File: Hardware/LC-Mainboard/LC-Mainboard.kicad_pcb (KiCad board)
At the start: 2 copper layers, 103 x 63 mm, 2 parts, among them J1 Raspberry_Pi, J2 Charge Controller

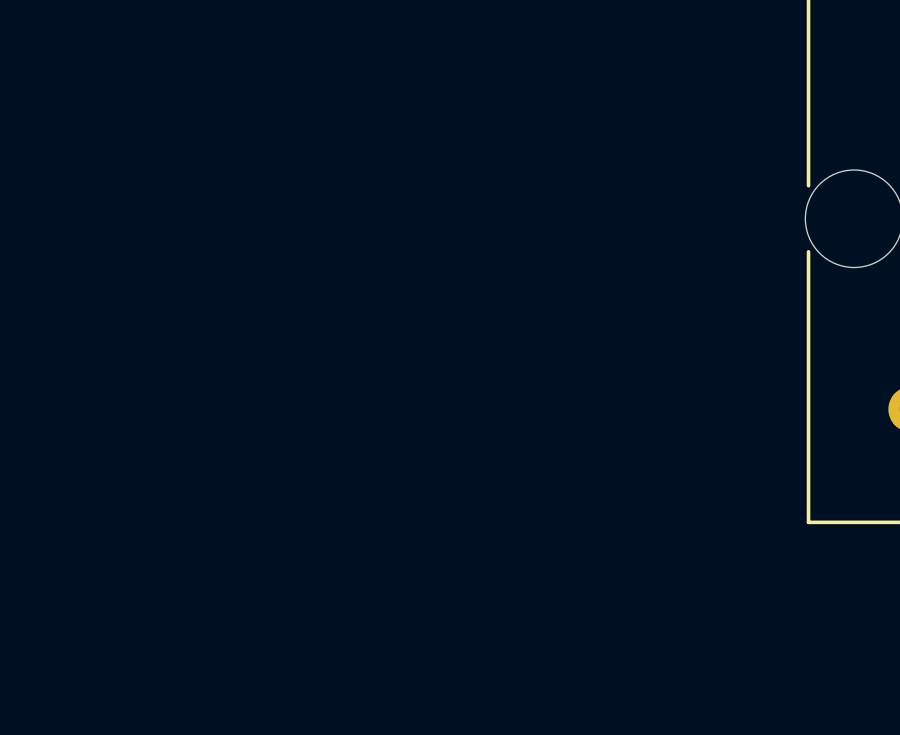
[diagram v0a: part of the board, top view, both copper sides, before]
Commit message: Update all
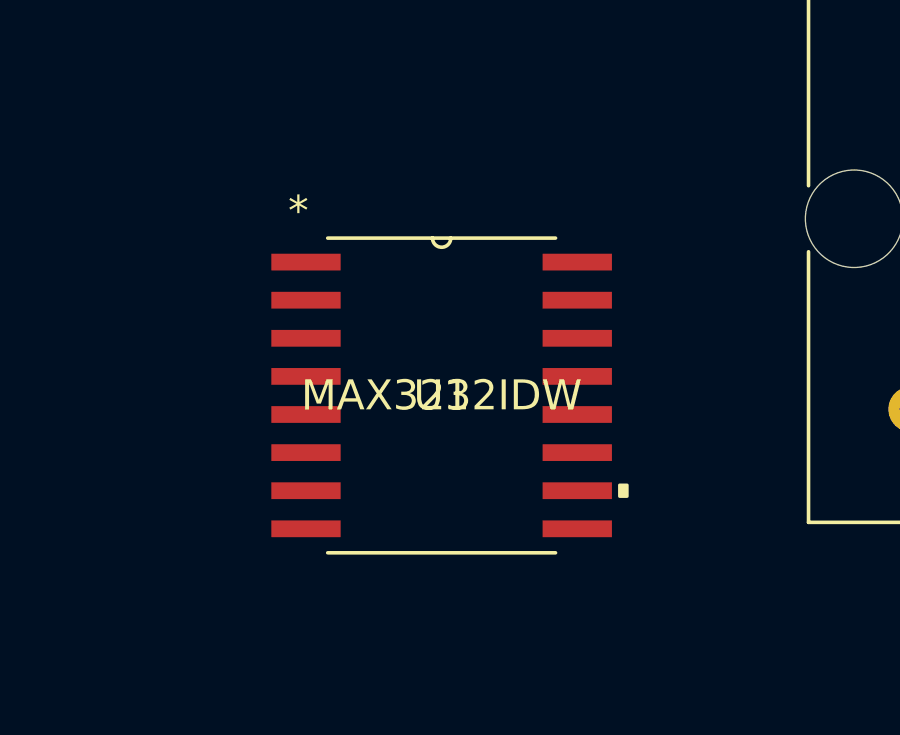
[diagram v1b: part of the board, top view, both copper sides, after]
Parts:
- added U1: MAX3232IDW, KenwoodFox:MAX3232IDW, F.Cu at (176.0, 86.0)
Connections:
- J2 pad 1: unconnected-(J2-Pad1) -> REN_TX
- J2 pad 2: unconnected-(J2-Pad2) -> REN_RX
- J2 pad 3: unconnected-(J2-Pad3) -> GND
